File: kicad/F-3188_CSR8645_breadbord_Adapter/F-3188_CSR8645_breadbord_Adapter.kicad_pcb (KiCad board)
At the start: 2 copper layers, 26.3 x 56.9 mm, 4 parts, among them J1 SCJ368R1NUS0B00G, P1 CONN_01X22, P2 CONN_01X21, U1 F-3188_CSR8645

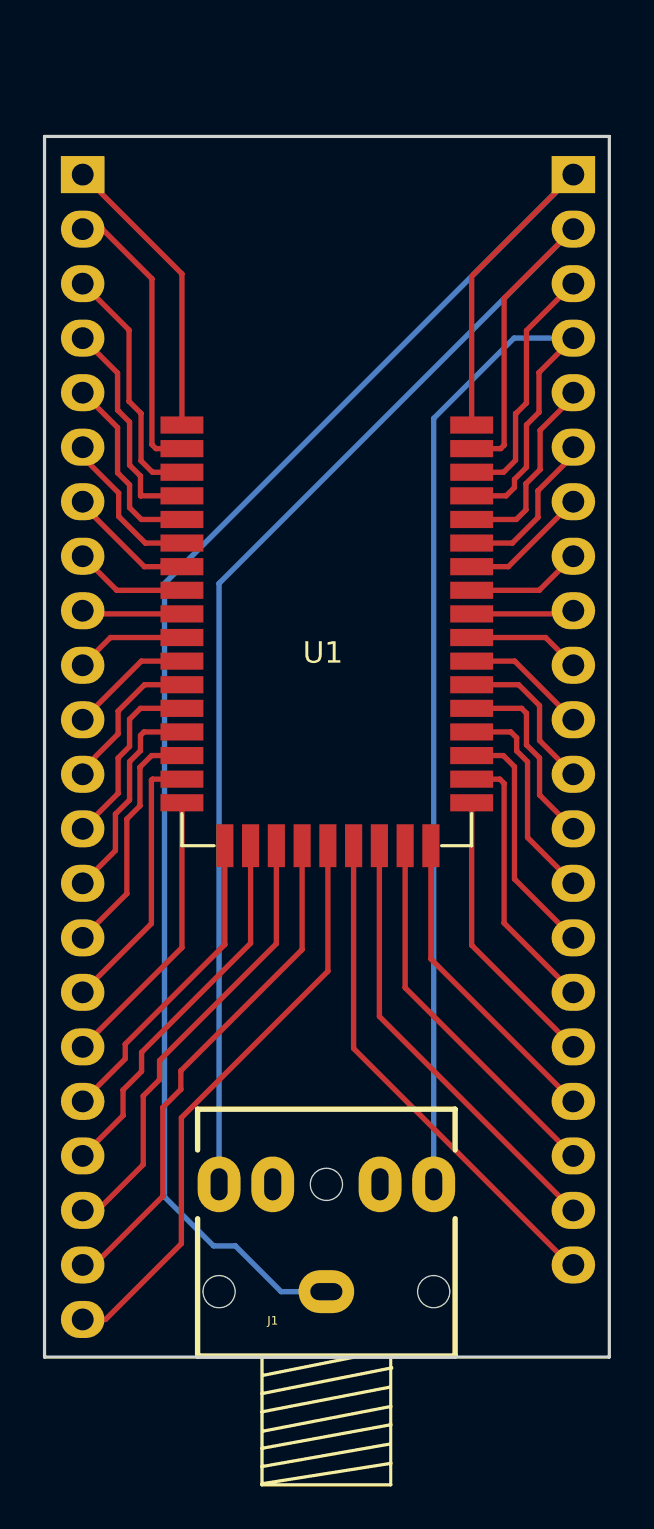
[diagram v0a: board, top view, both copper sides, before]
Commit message: updates
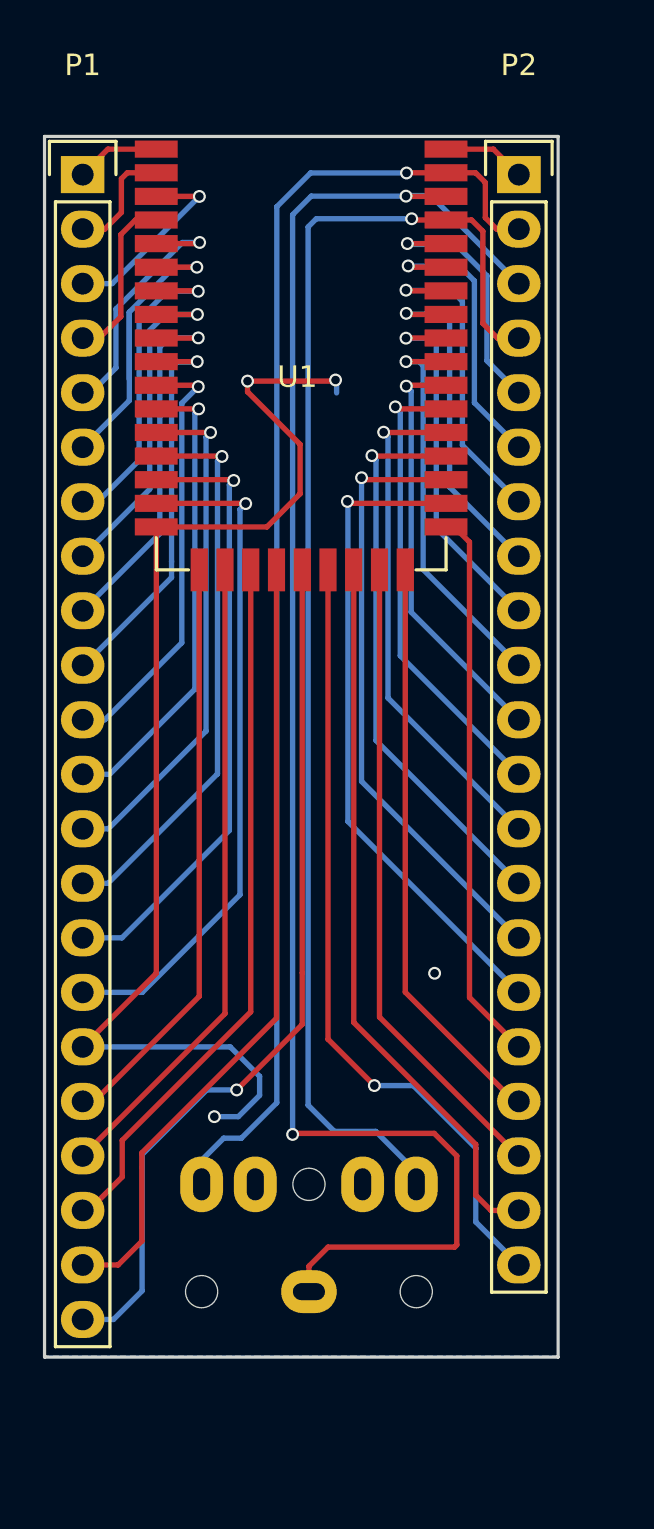
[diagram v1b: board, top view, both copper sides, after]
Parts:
- J1: footprint jacks:3.5mm_stereo_jack_PJ306M -> jacks:3.5mm_stereo_jack_PJ306M_no_screw_terminal; moved to B.Cu
- P1, P2: moved to F.Cu
- moved U1 12.9 mm to (138.0, 87.0)
- moved P2 2.54 mm to (154.9, 68.6), turned to 0 degrees
- moved J1 0.81 mm to (145.2, 120.6), turned to 0 degrees
- turned P1 to 0 degrees
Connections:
- net Net-(P1-Pad17) renamed /GND
- P2 pad 1: Net-(J1-Pad1) -> Net-(P2-Pad1)
- P2 pad 2: Net-(J1-Pad2) -> Net-(J1-Pad5)
- P2 pad 3: Net-(P2-Pad3) -> Net-(J1-Pad1)
- P2 pad 4: Net-(J1-Pad5) -> Net-(J1-Pad2)
- U1 pad 40: Net-(J1-Pad5) -> Net-(J1-Pad2)
- U1 pad 41: Net-(P2-Pad3) -> Net-(J1-Pad1)
- U1 pad 42: Net-(J1-Pad2) -> Net-(J1-Pad5)
- U1 pad 43: Net-(J1-Pad1) -> Net-(P2-Pad1)
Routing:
- net /GND: track 13.3 -> 56.2 mm, vias 0 -> 3
- net Net-(P1-Pad16): track 12.7 -> 31.7 mm, vias 0 -> 1
- net Net-(P2-Pad16): track 12.7 -> 30.8 mm, vias 0 -> 1
- net Net-(P1-Pad15): track 11.2 -> 28.9 mm, vias 0 -> 1
- net Net-(P2-Pad15): track 11.3 -> 28.5 mm, vias 0 -> 1
- net Net-(P1-Pad14): track 10.0 -> 26.3 mm, vias 0 -> 1
- net Net-(P2-Pad14): track 10.1 -> 26.2 mm, vias 0 -> 1
- net Net-(P1-Pad13): track 8.66 -> 24.2 mm, vias 0 -> 1
- net Net-(P2-Pad13): track 8.94 -> 24.0 mm, vias 0 -> 1
- net Net-(P1-Pad12): track 7.11 -> 22.0 mm, vias 0 -> 1
- net Net-(P1-Pad11): track 5.75 -> 20.3 mm, vias 0 -> 1
- net Net-(P2-Pad12): track 7.42 -> 21.9 mm, vias 0 -> 1
- net Net-(P2-Pad11): track 5.87 -> 19.6 mm, vias 0 -> 1
- net Net-(P1-Pad10): track 5.16 -> 18.8 mm, vias 0 -> 1
- net Net-(P1-Pad22): track 27.4 -> 40.8 mm, vias 0 -> 1
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- added copper zone on B.Cu, net /GND
- added copper zone on F.Cu, net /GND
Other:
- board size 26.3 x 56.9 mm -> 23.9 x 56.9 mm
